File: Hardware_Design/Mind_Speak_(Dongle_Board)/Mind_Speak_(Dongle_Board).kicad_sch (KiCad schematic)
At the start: 3 parts, among them J1 USB_A, SW1 SPDT_Slide_SMD_6.7x2.6mm, U1 FT231XQ

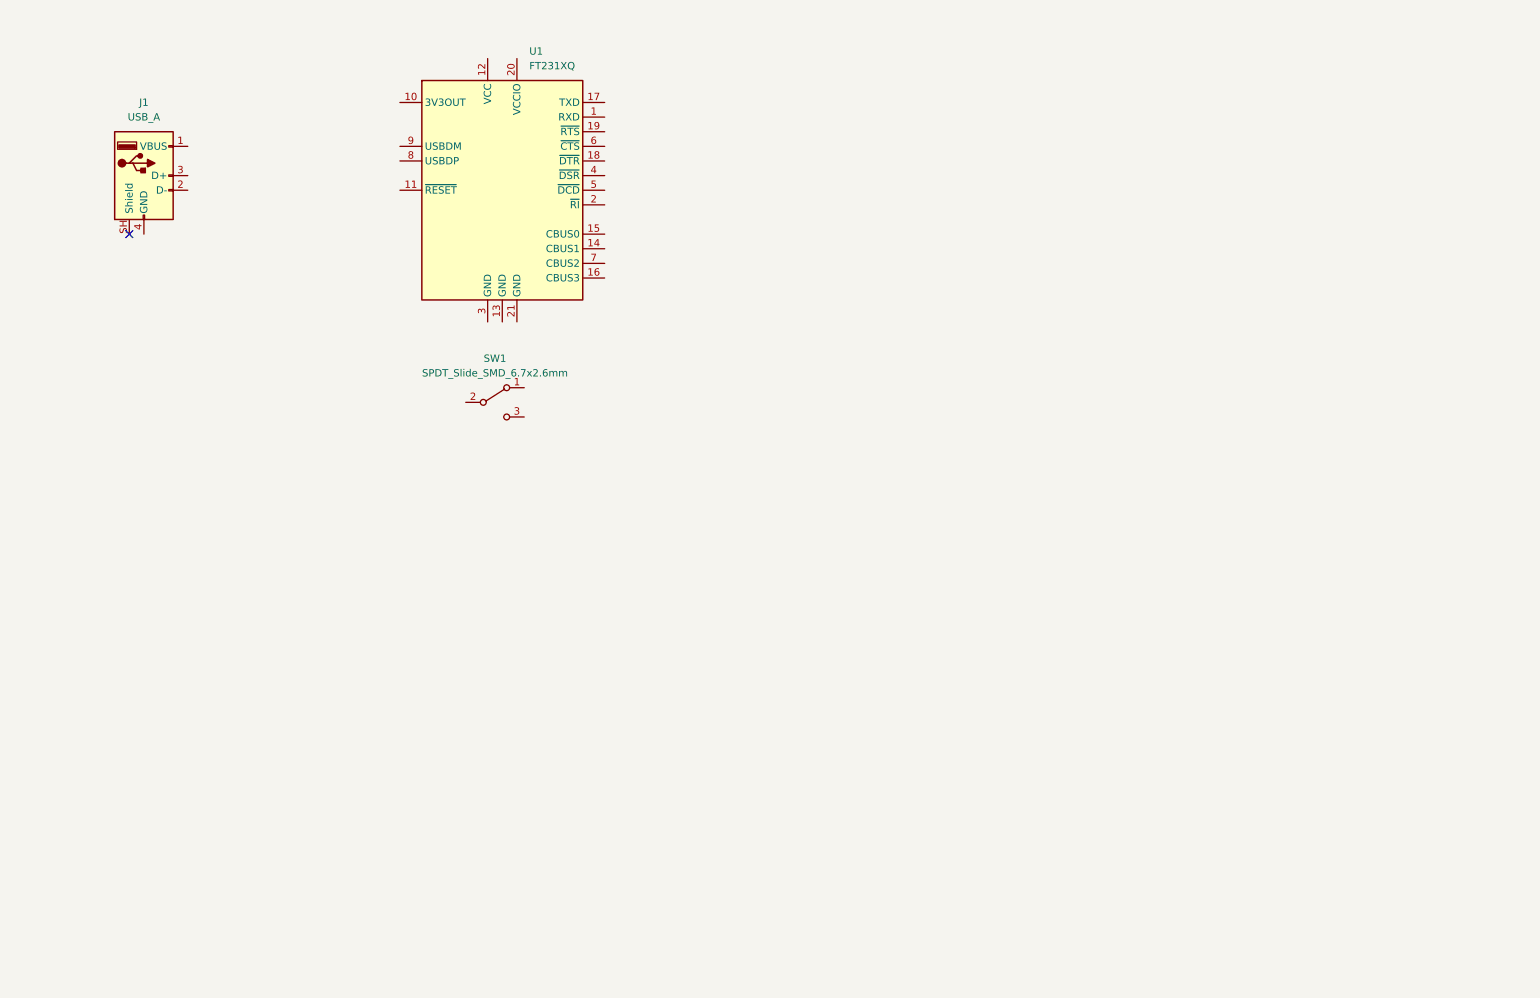
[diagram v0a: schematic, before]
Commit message: Edit In Dongle Board
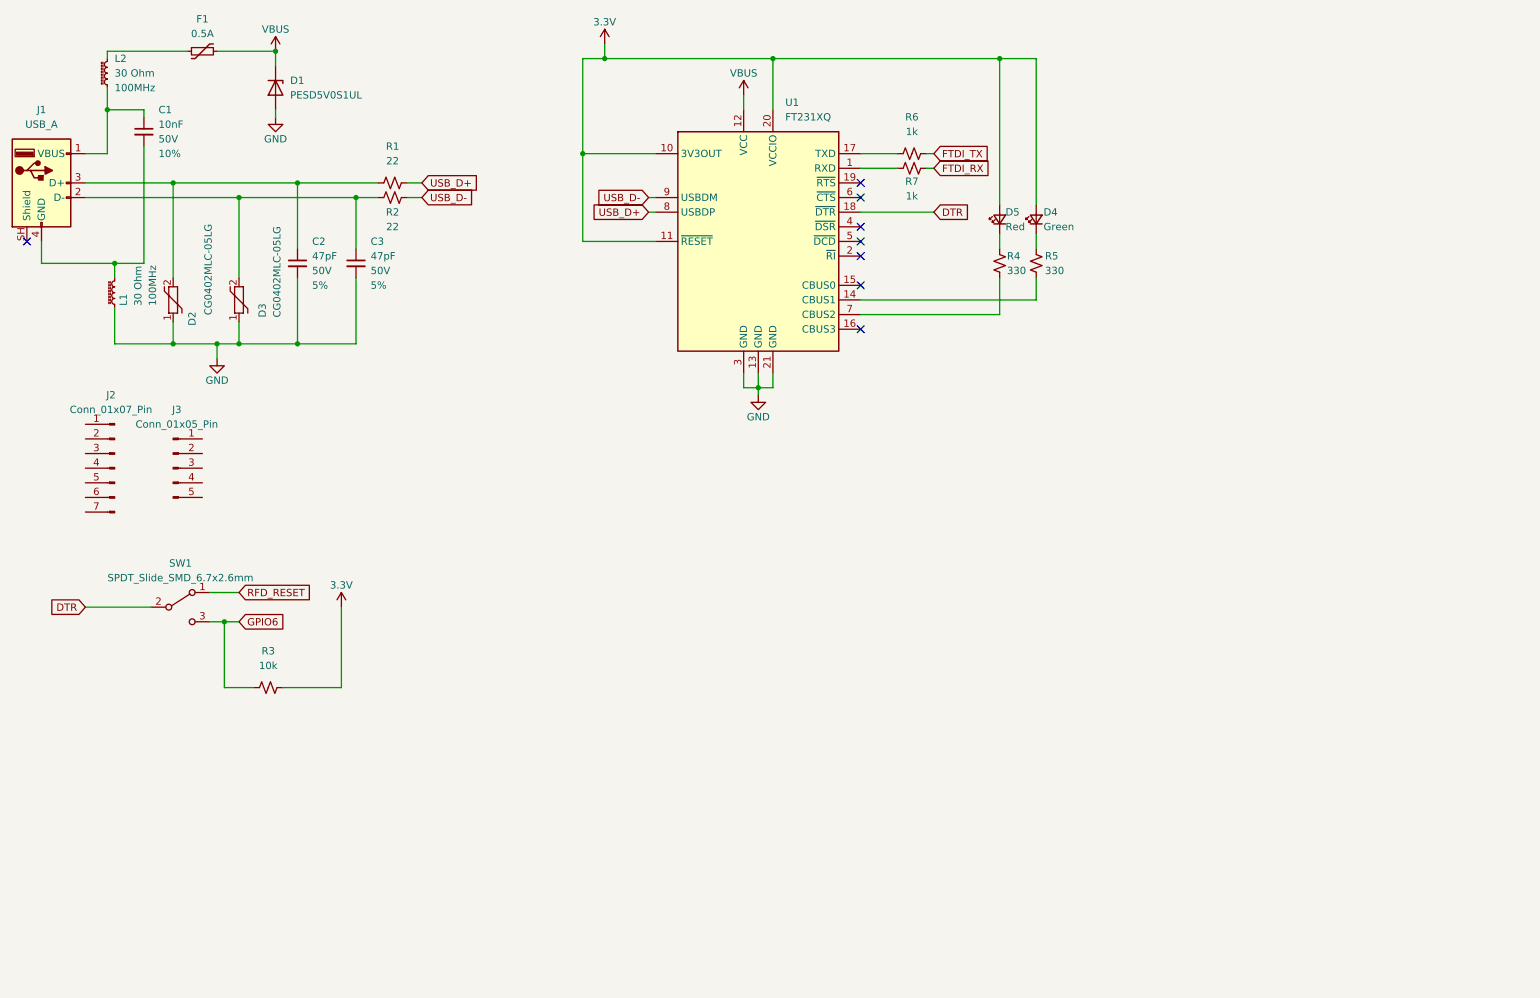
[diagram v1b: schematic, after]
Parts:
- added C1: 10nF, PCM_SparkFun-Capacitor:C_0402_1005Metric, symbol PCM_SparkFun-Capacitor:10nF_0402_25V_10%
- added C2, C3: 47pF, Capacitors SMD:CAPC0603X33N, symbol PCM_SparkFun-Capacitor:47pF_0603_50V_5%
- added D1: PESD5V0S1UL, Diode_SMD:D_SOD-882, symbol Diode:PESD5V0S1UL
- added D2, D3: CG0402MLC-05LG, ESD_SMD:CG0402MLC-05LG, symbol Device:CG0402MLC-05LG
- added D4: Green, PCM_SparkFun-LED:LED_0603_1608Metric_Green, symbol PCM_SparkFun-LED:LED_Green_0603
- added D5: Red, PCM_SparkFun-LED:LED_0603_1608Metric_Red, symbol PCM_SparkFun-LED:LED_Red_0603
- added F1: 0.5A, PCM_SparkFun-Fuse:1812, symbol PCM_SparkFun-Fuse:Fuse 16V/2.5A/5.0A
- added J2: Conn_01x07_Pin, Connector_PinHeader_2.54mm:PinHeader_1x07_P2.54mm_Vertical, symbol Connector:Conn_01x07_Pin
- added J3: Conn_01x05_Pin, Connector_PinHeader_2.54mm:PinHeader_1x05_P2.54mm_Vertical, symbol Connector:Conn_01x05_Pin
- added L1, L2: 30 Ohm, PCM_SparkFun-Capacitor:C_0402_1005Metric, symbol PCM_SparkFun-Coil:Ferrite_120Ohm_0402_0.3A
- added R1, R2: 22, PCM_SparkFun-Resistor:R_0402_1005Metric, symbol PCM_SparkFun-Resistor:22_0402
- added R3: 10k, PCM_SparkFun-Resistor:R_0402_1005Metric, symbol PCM_SparkFun-Resistor:10k_0402
- added R4, R5: 330, PCM_SparkFun-Resistor:R_0402_1005Metric, symbol PCM_SparkFun-Resistor:330_0402
- added R6, R7: 1k, PCM_SparkFun-Resistor:R_0402_1005Metric, symbol PCM_SparkFun-Resistor:1k_0402
- J1: footprint (none) -> Connector_USB:MOLEX_48037-1000
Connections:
- net at J1.1 (VBUS): now also C1.1, L2.1
- net at J1.2 (D-): now also C3.1, D3.2, R2.1
- net at J1.3 (D+): now also C2.1, D2.2, R1.1
- net at J1.4 (GND): now also C1.2, L1.2
- net at U1.1 (RXD): now also R7.1
- net 3.3V: now reaches U1.10 (3V3OUT)
- net 3.3V: now also U1.11 (~{RESET}), U1.20 (VCCIO), D4.2 (A), D5.2 (A), R3.2
- net VBUS: now reaches U1.12 (VCC)
- net VBUS: now also D1.1 (K), F1.2
- net GND: now reaches U1.13 (GND)
- net GND: now also U1.21 (GND), U1.3 (GND), C2.2, C3.2, D1.2 (A), D2.1, D3.1, L1.1
- net at U1.14 (CBUS1): now also R5.1
- net at U1.17 (TXD): now also R6.1
- net DTR: now reaches U1.18 (~{DTR})
- net DTR: now also SW1.2
- net at U1.7 (CBUS2): now also R4.1
- net USB_D+: now reaches U1.8 (USBDP)
- net USB_D+: now also R1.2
- net USB_D-: now reaches U1.9 (USBDM)
- net USB_D-: now also R2.2
- net RFD_RESET: now reaches SW1.1 (A)
- net GPIO6: now reaches SW1.3 (C)
- net GPIO6: now also R3.1
- new net: D5.1 (K), R4.2
- new net: F1.1, L2.2
- new net: D4.1 (K), R5.2
- new net FTDI_RX: R7.2
- new net FTDI_TX: R6.2
- no-connect marks 1 -> 8
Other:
- moved on the sheet: J1, SW1, U1

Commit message: Edit The main Board
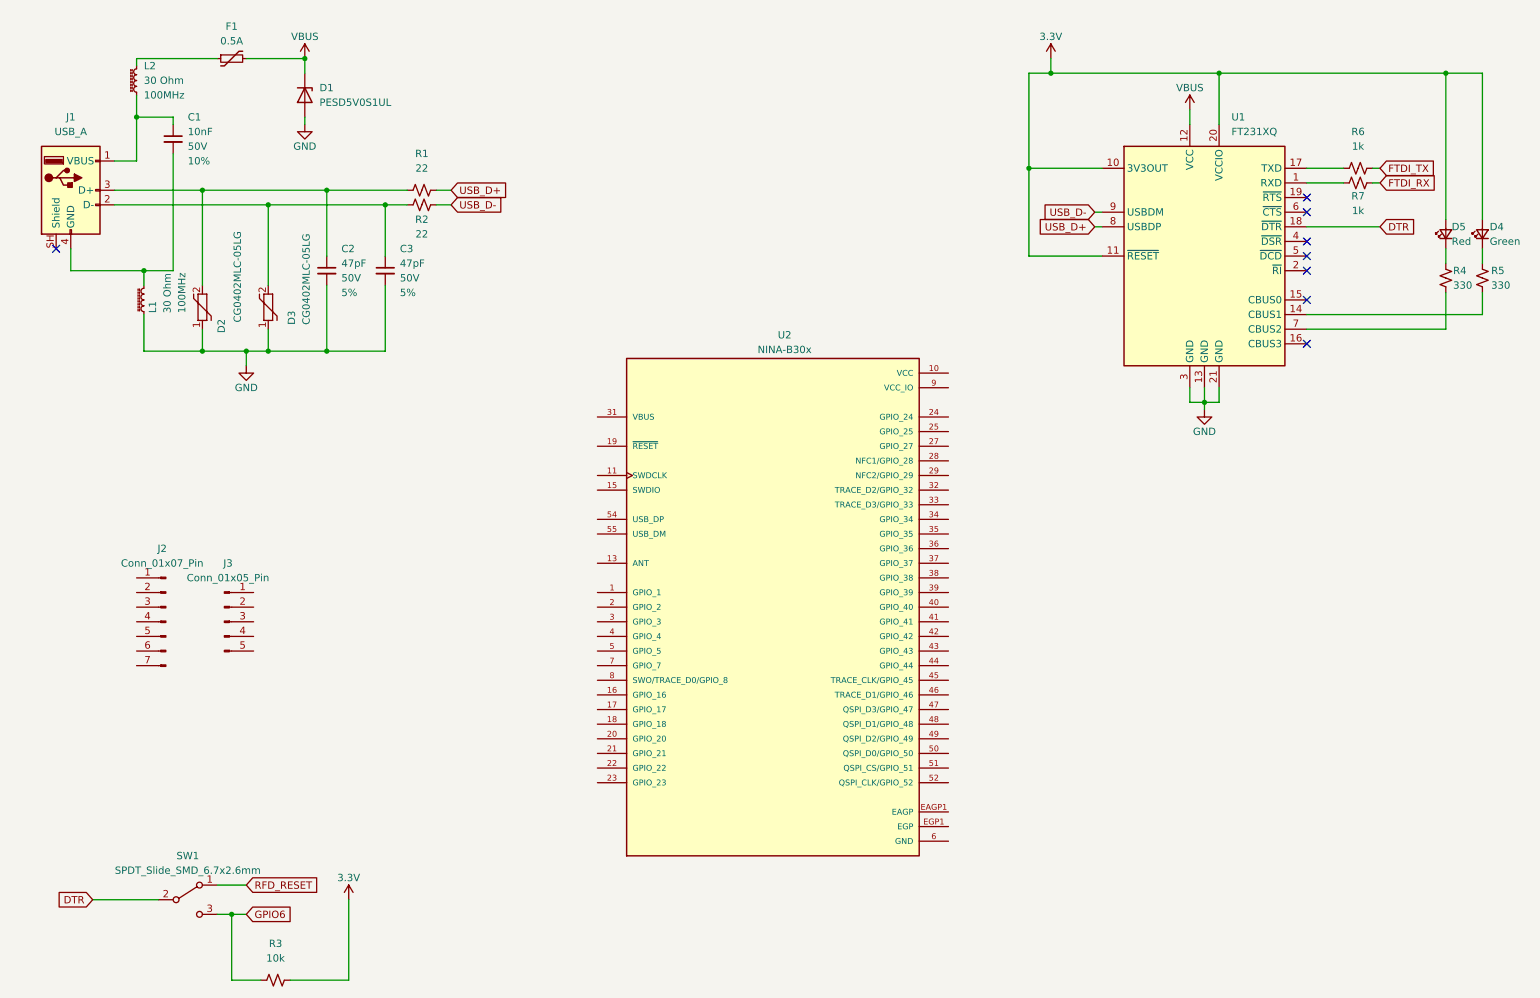
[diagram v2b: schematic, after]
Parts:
- added U2: NINA-B30x, U_Blox_Library:XCVR_NINA-B306-00B, symbol NINA-B306-00B:NINA-B30x
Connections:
- net GND: now also U2.12 (GND), U2.14 (GND), U2.26 (GND), U2.30 (GND), U2.53 (GND), U2.6 (GND)
- new net EAGP: U2.EAGP1 (EAGP), U2.EAGP2 (EAGP), U2.EAGP3 (EAGP), U2.EAGP4 (EAGP)
- new net EGP: U2.EGP1 (EGP), U2.EGP10 (EGP), U2.EGP11 (EGP), U2.EGP12 (EGP), U2.EGP2 (EGP), U2.EGP3 (EGP), U2.EGP4 (EGP), U2.EGP5 (EGP), U2.EGP6 (EGP), U2.EGP7 (EGP), U2.EGP8 (EGP), U2.EGP9 (EGP)
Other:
- moved on the sheet: C1, C2, C3, D1, D2, D3, D4, D5, F1, J1, J2, J3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
